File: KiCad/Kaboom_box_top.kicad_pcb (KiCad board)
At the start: 2 copper layers, 150 x 140 mm, 83 parts, among them J130 2mm_clamp, J131 2mm_clamp, J132 2mm_clamp, J133 2mm_clamp, J134 2mm_clamp, J135 2mm_clamp, J136 2mm_clamp, J137 2mm_clamp, J138 2mm_clamp, J139 2mm_clamp, J140 2mm_clamp, J141 2mm_clamp, J142 2mm_clamp, J143 2mm_clamp, J144 2mm_clamp, J145 2mm_clamp, J146 2mm_clamp, J147 2mm_clamp, J148 2mm_clamp, J149 2mm_clamp, J150 2mm_clamp, J151 2mm_clamp, J152 2mm_clamp, J153 2mm_clamp, J154 2mm_clamp, J155 2mm_clamp, J156 2mm_clamp, J157 2mm_clamp, J158 2mm_clamp, P101 HDR-IDC-2_54-2X5P, P103 HDR-IDC-2_54-2X5P, P105 HDR-IDC-2_54-2X5P, U144 HS96L03W2C03, U145 74HC165D,653, U146 74HC165D,653, U147 74HC165D,653, U148 74HC165D,653, U150 WS2812E-MINI-X1, U151 WS2812E-MINI-X1, U152 WS2812E-MINI-X1, U153 WS2812E-MINI-X1, U154 WS2812E-MINI-X1, U155 WS2812E-MINI-X1, U156 WS2812E-MINI-X1, U157 WS2812E-MINI-X1, U158 WS2812E-MINI-X1, U159 WS2812E-MINI-X1, U160 WS2812E-MINI-X1, U161 WS2812E-MINI-X1, U162 WS2812E-MINI-X1, U163 WS2812E-MINI-X1, U164 WS2812E-MINI-X1, U165 WS2812E-MINI-X1, U166 WS2812E-MINI-X1, U167 WS2812E-MINI-X1, U168 WS2812E-MINI-X1, U169 WS2812E-MINI-X1, U170 WS2812E-MINI-X1, U171 WS2812E-MINI-X1, U172 WS2812E-MINI-X1, U173 WS2812E-MINI-X1, U174 WS2812E-MINI-X1, U175 WS2812E-MINI-X1, U176 WS2812E-MINI-X1, U177 WS2812E-MINI-X1, U178 WS2812E-MINI-X1

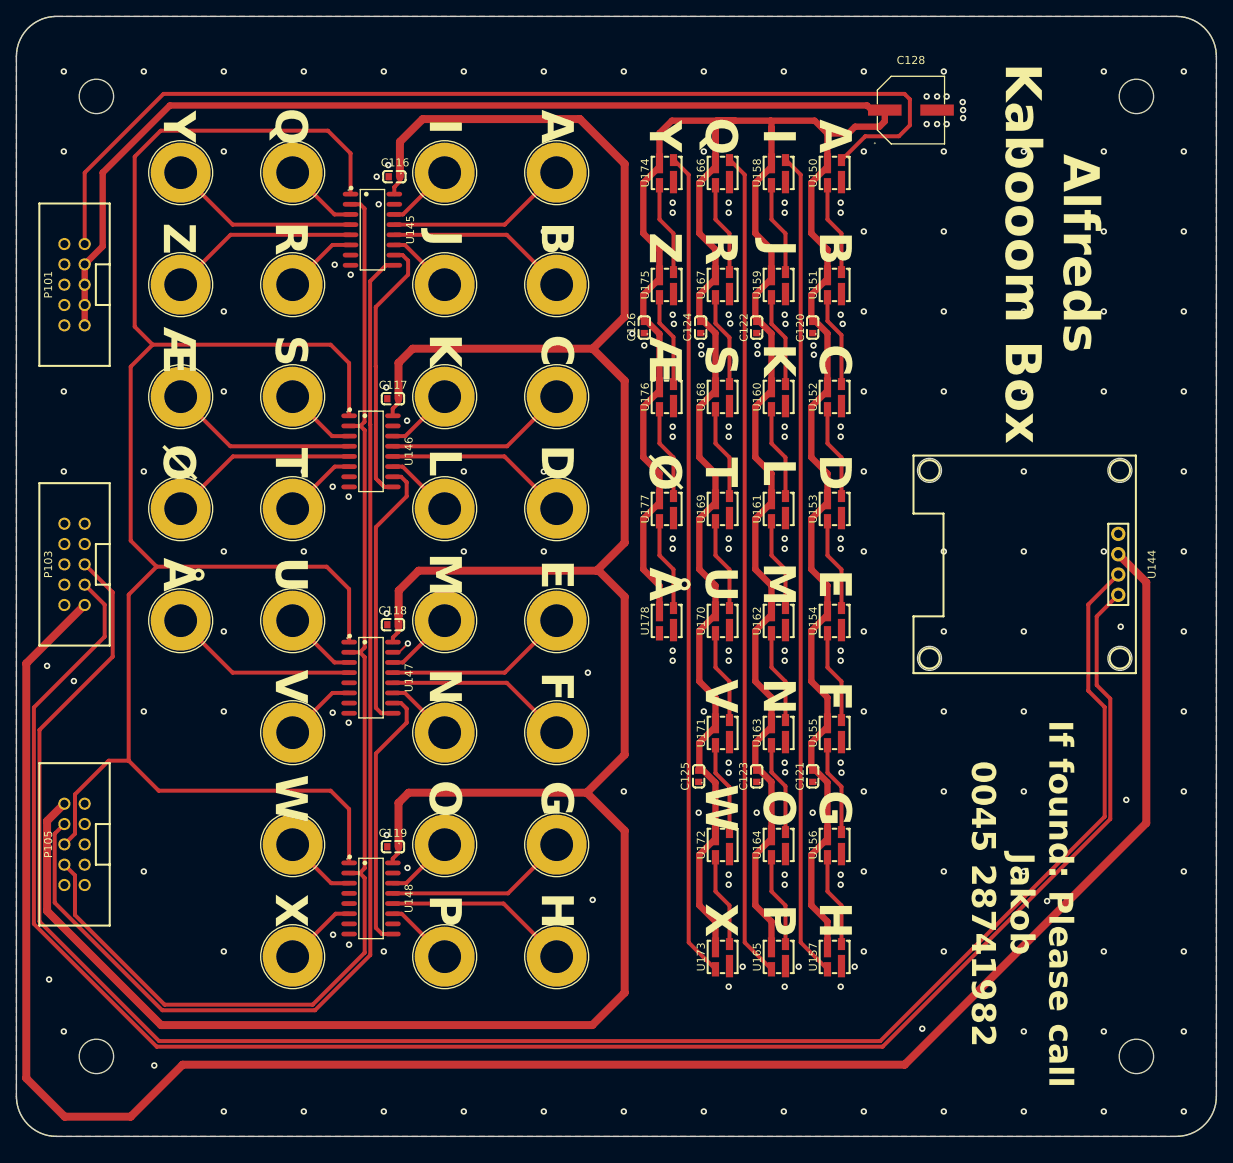
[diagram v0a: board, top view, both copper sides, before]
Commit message: Updates for V2
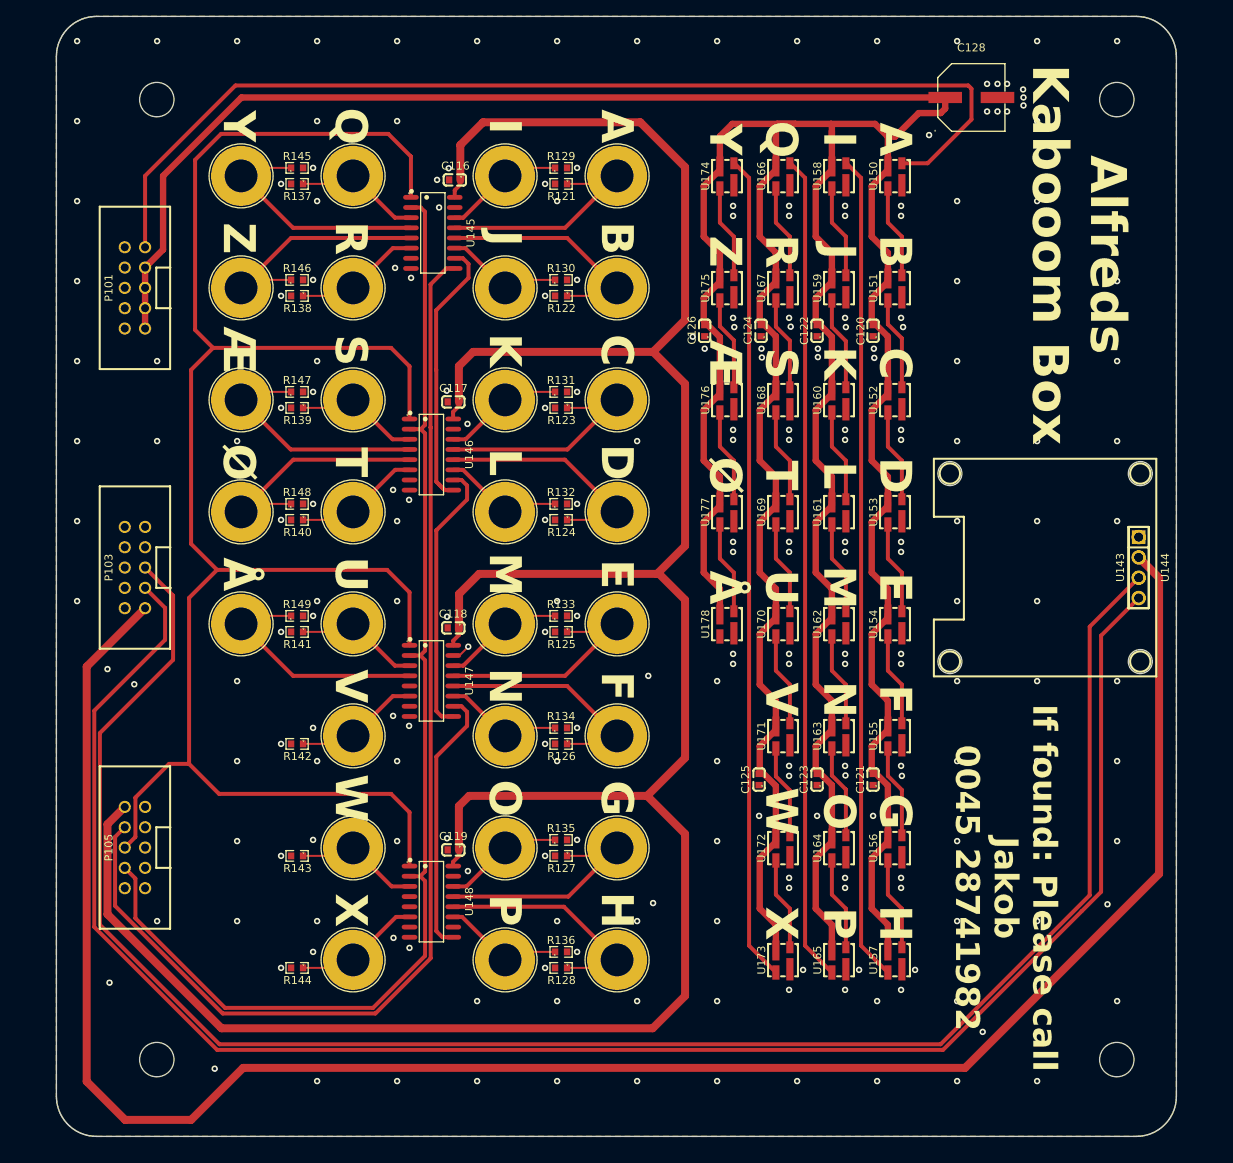
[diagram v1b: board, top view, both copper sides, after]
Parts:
- added R121: 0603WAF1202T5E, footprint:R0603, F.Cu at (203.1, 40.9)
- added R122: 0603WAF1202T5E, footprint:R0603, F.Cu at (203.1, 54.9)
- added R123: 0603WAF1202T5E, footprint:R0603, F.Cu at (203.1, 68.9)
- added R124: 0603WAF1202T5E, footprint:R0603, F.Cu at (203.1, 82.9)
- added R125: 0603WAF1202T5E, footprint:R0603, F.Cu at (203.1, 96.9)
- added R126: 0603WAF1202T5E, footprint:R0603, F.Cu at (203.1, 110.9)
- added R127: 0603WAF1202T5E, footprint:R0603, F.Cu at (203.1, 124.9)
- added R128: 0603WAF1202T5E, footprint:R0603, F.Cu at (203.1, 138.9)
- added R129: 0603WAF1202T5E, footprint:R0603, F.Cu at (203.1, 38.9)
- added R130: 0603WAF1202T5E, footprint:R0603, F.Cu at (203.1, 52.9)
- added R131: 0603WAF1202T5E, footprint:R0603, F.Cu at (203.1, 66.9)
- added R132: 0603WAF1202T5E, footprint:R0603, F.Cu at (203.1, 80.9)
- added R133: 0603WAF1202T5E, footprint:R0603, F.Cu at (203.1, 94.9)
- added R134: 0603WAF1202T5E, footprint:R0603, F.Cu at (203.1, 108.9)
- added R135: 0603WAF1202T5E, footprint:R0603, F.Cu at (203.1, 122.9)
- added R136: 0603WAF1202T5E, footprint:R0603, F.Cu at (203.1, 136.9)
- added R137: 0603WAF1202T5E, footprint:R0603, F.Cu at (170.1, 40.9)
- added R138: 0603WAF1202T5E, footprint:R0603, F.Cu at (170.1, 54.9)
- added R139: 0603WAF1202T5E, footprint:R0603, F.Cu at (170.1, 68.9)
- added R140: 0603WAF1202T5E, footprint:R0603, F.Cu at (170.1, 82.9)
- added R141: 0603WAF1202T5E, footprint:R0603, F.Cu at (170.1, 96.9)
- added R142: 0603WAF1202T5E, footprint:R0603, F.Cu at (170.1, 110.9)
- added R143: 0603WAF1202T5E, footprint:R0603, F.Cu at (170.1, 124.9)
- added R144: 0603WAF1202T5E, footprint:R0603, F.Cu at (170.1, 138.9)
- added R145: 0603WAF1202T5E, footprint:R0603, F.Cu at (170.1, 38.9)
- added R146: 0603WAF1202T5E, footprint:R0603, F.Cu at (170.1, 52.9)
- added R147: 0603WAF1202T5E, footprint:R0603, F.Cu at (170.1, 66.9)
- added R148: 0603WAF1202T5E, footprint:R0603, F.Cu at (170.1, 80.9)
- added R149: 0603WAF1202T5E, footprint:R0603, F.Cu at (170.1, 94.9)
- added U143: PZ254V-11-04P_C2691448, footprint:HDR-TH_4P-P2.54-V-M, F.Cu at (275.3, 88.9)
- moved C128 7.71 mm to (254.4, 30.1)
- moved C117 7.56 mm to (189.6, 68.2)
- moved C118 7.56 mm to (189.6, 96.4)
- moved C119 7.56 mm to (189.6, 124.2)
- moved C121 7.56 mm to (242.1, 115.4)
- moved C123 7.56 mm to (235.1, 115.4)
- moved C125 7.56 mm to (227.8, 115.4)
- moved H108 7.56 mm to (152.5, 150.4)
- moved J132 7.56 mm to (210.1, 67.9)
- moved J133 7.56 mm to (210.1, 81.9)
- moved J134 7.56 mm to (210.1, 95.9)
- moved J135 7.56 mm to (210.1, 109.9)
- moved J136 7.56 mm to (210.1, 123.9)
- moved J140 7.56 mm to (196.1, 67.9)
- moved J141 7.56 mm to (196.1, 81.9)
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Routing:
- net Board_0-/Top/Shift_Parallel_to_Serial/J146: track 9.40 -> 16.1 mm
- net Board_0-/Top/Shift_Parallel_to_Serial/J138: track 8.46 -> 15.1 mm
- net Board_0-/Top/Shift_Parallel_to_Serial/J157: track 23.8 -> 30.4 mm
- net Board_0-/Top/Shift_Parallel_to_Serial/J154: track 23.9 -> 30.6 mm
- net Board_0-/Top/Shift_Parallel_to_Serial/J151: track 9.11 -> 15.8 mm
- net Board_0-/Top/Shift_Parallel_to_Serial/J149: track 9.23 -> 15.9 mm
- net Board_0-/Top/Shift_Parallel_to_Serial/J147: track 9.29 -> 16.0 mm
- net Board_0-/Top/Shift_Parallel_to_Serial/J143: track 8.53 -> 15.2 mm
- net Board_0-/Top/Shift_Parallel_to_Serial/J141: track 8.65 -> 15.3 mm
- net Board_0-/Top/Shift_Parallel_to_Serial/J139: track 8.35 -> 15.0 mm
- net Board_0-/Top/Shift_Parallel_to_Serial/J136: track 23.0 -> 29.7 mm
- net Board_0-/Top/Shift_Parallel_to_Serial/J135: track 23.1 -> 29.7 mm
- net Board_0-/Top/Shift_Parallel_to_Serial/J133: track 23.2 -> 29.8 mm
- net Board_0-/Top/Shift_Parallel_to_Serial/J130: track 23.0 -> 29.6 mm
- net Board_0-/Top/Shift_Parallel_to_Serial/J156: track 23.6 -> 30.3 mm
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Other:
- board size 150 x 140 mm -> 140 x 140 mm
